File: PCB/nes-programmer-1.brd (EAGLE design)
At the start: 130 x 50 mm, 32 parts, among them J3 Molex 22-28-8062, M1 ATmega328P Module, M2 0124A, SW1 Push Switch, U1 MCP23S08, U2 MCP23S17

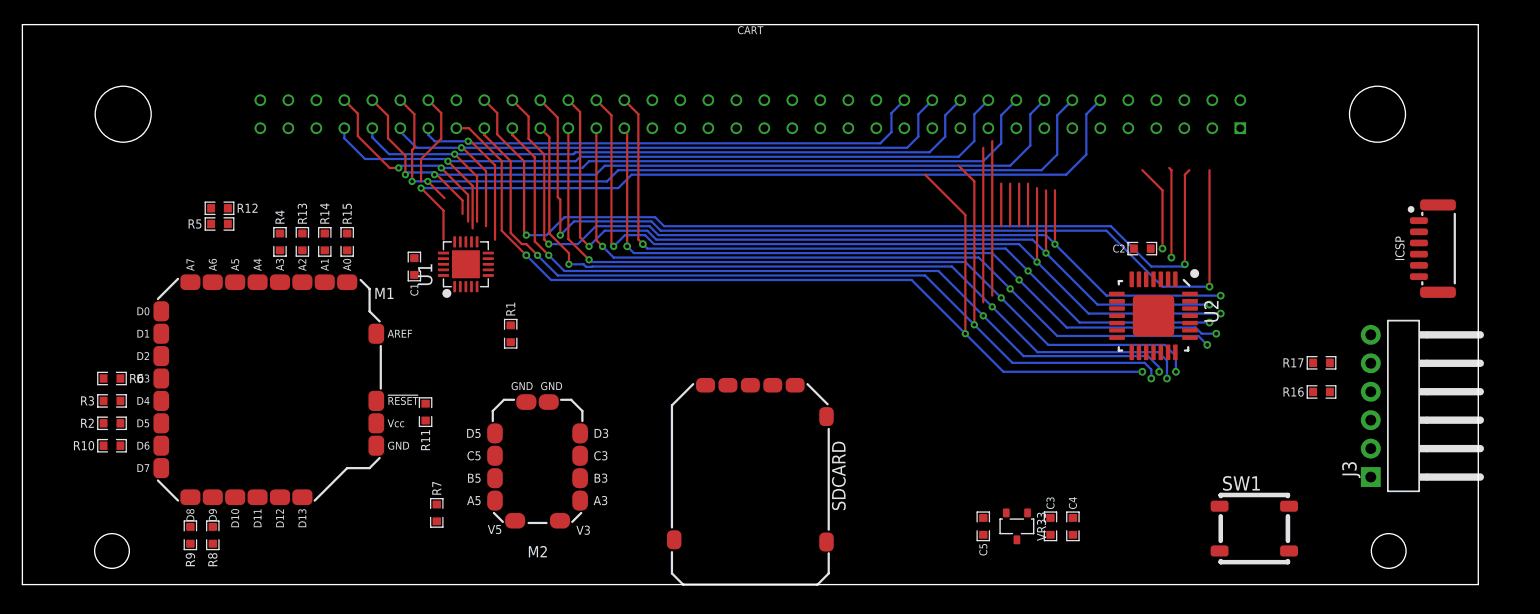
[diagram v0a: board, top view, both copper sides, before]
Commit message: Final tweaks.
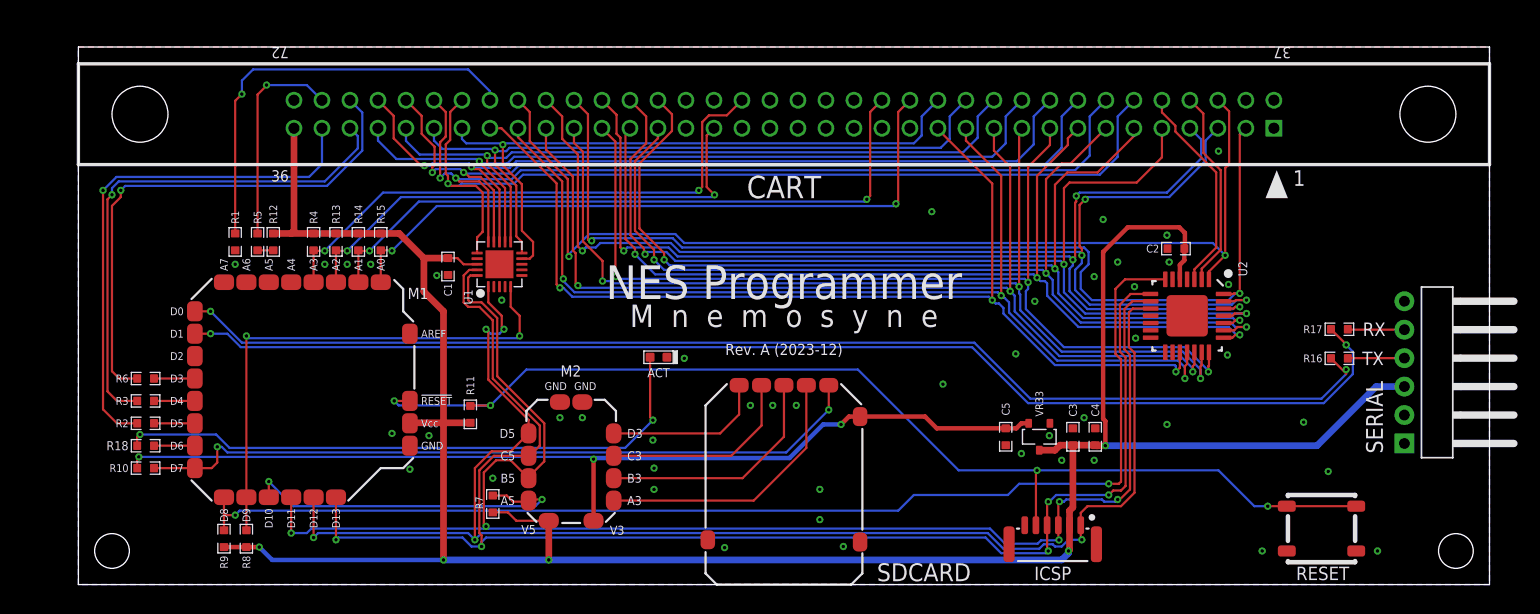
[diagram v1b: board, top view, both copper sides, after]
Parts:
- removed J3: Molex 22-28-8062, con-headers:MA06X1-RA-THD
- removed SW1: Push Switch, switch-smd:B3SN
- added ACT: (no value), led:SMD_0603
- added R18: 2K, rlc:0603-RES
- added RESET: Push Switch, switch-smd:B3SN
- added SERIAL: Molex 22-28-8062, con-headers:MA06X1-RA-THD
- moved ICSP 41.4 mm to (87.0, 5.00), turned to 180 degrees
- moved R1 25.9 mm to (14.0, 30.6)
- moved C3 8.25 mm to (88.8, 13.2)
- moved C4 8.25 mm to (90.8, 13.2)
- moved C5 8.25 mm to (82.8, 13.2)
- moved VR33 8.25 mm to (85.8, 13.2)
- moved R12 5.66 mm to (17.4, 30.6), turned to 90 degrees
- moved R7 5.06 mm to (37.0, 7.20), turned to 270 degrees
- moved R11 4.00 mm to (35.0, 15.2)
- moved R5 3.76 mm to (16.0, 30.6), turned to 270 degrees
- moved R10 3.61 mm to (6.00, 10.4)
- moved R16 3.40 mm to (112.6, 20.2)
- moved R17 3.40 mm to (112.6, 22.8)
- moved R8 3.01 mm to (15.0, 4.10)
- moved R9 3.01 mm to (13.0, 4.10)
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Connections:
- new net ACTIVITY: M1.D6, R18.1
- new net ACT_LED: ACT.A, R18.2
- net !RESET: now also RESET.3, RESET.4; no longer SW1.3, SW1.4
- net FT_RX: now also SERIAL.5; no longer J3.5
- net FT_TX: now also SERIAL.4; no longer J3.4
- net GND: now also ACT.K, RESET.1, RESET.2, SERIAL.1; no longer J3.1, SW1.1, SW1.2
- net SD_!DET: now also M1.D7; no longer M1.D6
- net VCC: now also SERIAL.3; no longer J3.3
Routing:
- net VCC: track 0.00 -> 221.8 mm, vias 0 -> 5
- net SPI_MOSI: track 0.00 -> 134.9 mm, vias 0 -> 5
- net SPI_SCK: track 0.00 -> 133.7 mm, vias 0 -> 5
- net SPI_MISO: track 0.00 -> 130.0 mm, vias 0 -> 5
- net TX: track 0.00 -> 111.9 mm, vias 0 -> 2
- net RX: track 0.00 -> 109.6 mm, vias 0 -> 2
- net ADDR_!CS: track 0.00 -> 106.5 mm, vias 0 -> 2
- net !RESET: track 0.00 -> 100.6 mm, vias 0 -> 4
- net +3.3V: track 0.00 -> 88.3 mm, vias 0 -> 3
- net SD_!DET: track 0.00 -> 65.8 mm, vias 0 -> 2
- net PGM_!OE: track 0.00 -> 60.4 mm, vias 0 -> 2
- net PGM_!WR: track 0.00 -> 59.6 mm, vias 0 -> 2
- net ACT_LED: track 0.00 -> 54.2 mm, vias 0 -> 2
- net CHR_!WR: track 0.00 -> 50.1 mm, vias 0 -> 2
- net CIC_+RST: track 0.00 -> 47.0 mm, vias 0 -> 1
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- added copper zone on layer 1, net GND
- added copper zone on layer 16, net GND
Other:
- board size 130 x 50 mm -> 126 x 48 mm
- board text added: "M n e m o s y n e"
- board text added: "MNEMOSYNE"
- board text added: "NES Programmer"
- board text added: "RX"
- board text added: "Rev. A (2023-12)"
- board text added: "TX"
- board text added: "by Circuit Monkey"
